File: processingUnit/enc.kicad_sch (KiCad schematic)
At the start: 14 parts, among them J305 Conn_01x04, SW201 ENC RST, U201 STM32F103Cx, Y201 8Mhz

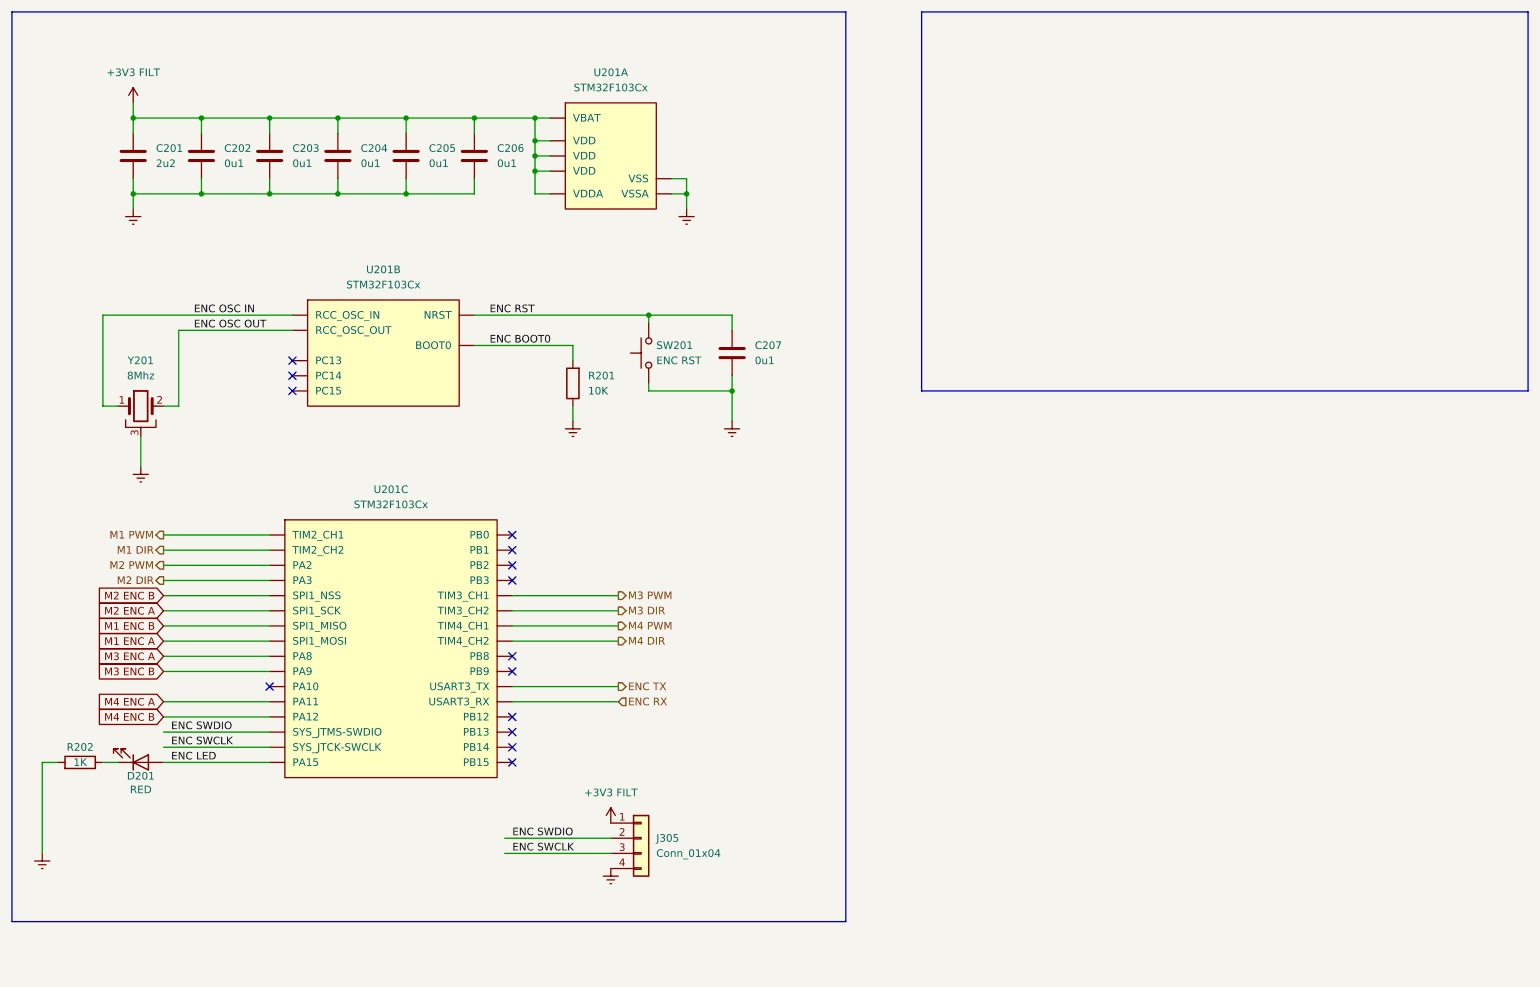
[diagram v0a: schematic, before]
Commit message: l3 might redo
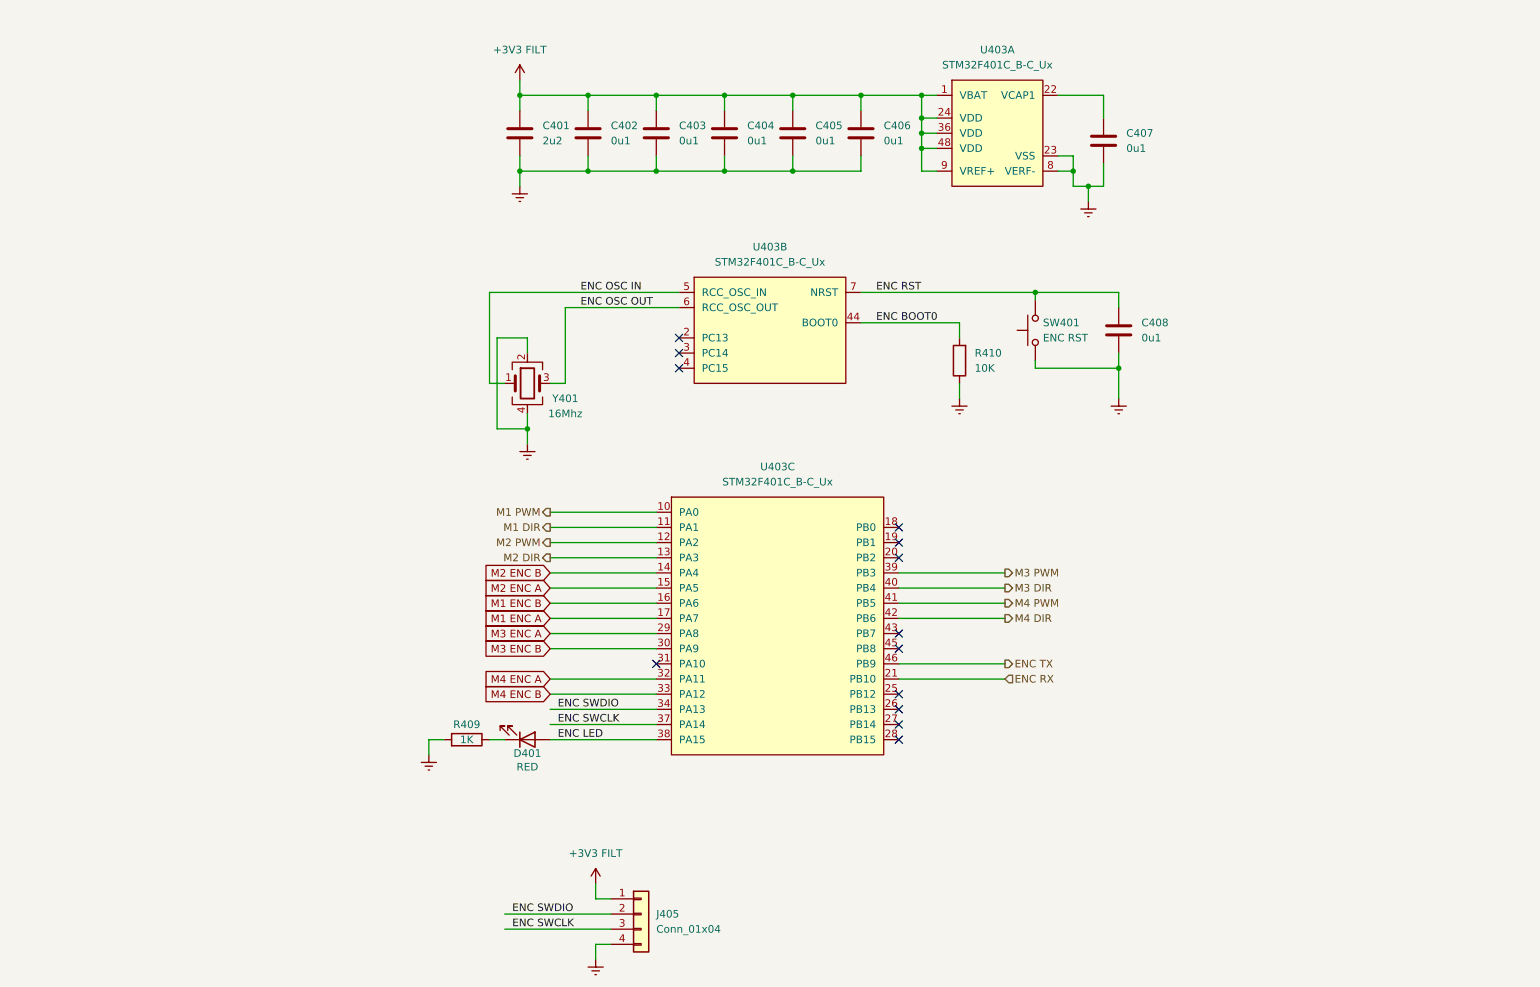
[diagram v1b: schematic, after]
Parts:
- removed U201: STM32F103Cx, Package_DFN_QFN:QFN-48-1EP_7x7mm_P0.5mm_EP5.6x5.6mm, symbol vincent:STM32F103Cx
- removed Y201: 8Mhz, Library:CSTCE8M00G52-R0, symbol Device:Crystal_GND3
- added C407: 0u1, Library:cap0603, symbol Device:C
- added U403: STM32F401C_B-C_Ux, Package_DFN_QFN:QFN-48-1EP_7x7mm_P0.5mm_EP5.6x5.6mm, symbol vincent:STM32F401C_B-C_Ux
- added Y401: 16Mhz, Library:CX3225SB16000D0FPLCC, symbol Device:Crystal_GND24
- renumbered C201 to C401, C202 to C402, C203 to C403, C204 to C404, C205 to C405, C206 to C406, C207 to C408, D201 to D401, J305 to J405, R202 to R409, R201 to R410, SW201 to SW401
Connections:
- net +3V3 FILT: now also U403.1 (VBAT), U403.24 (VDD), U403.36 (VDD), U403.48 (VDD), U403.9 (VREF+)
- net ENC BOOT0: now also U403.44 (BOOT0)
- net ENC LED: now also U403.38 (PA15)
- net ENC OSC IN: now also U403.5 (PH0), Y401.1
- net ENC OSC OUT: now also U403.6 (PH1), Y401.3
- net ENC RST: now also U403.7 (NRST)
- net ENC RX: now also U403.21 (PB10)
- net ENC SWCLK: now also U403.37 (PA14)
- net ENC SWDIO: now also U403.34 (PA13)
- net ENC TX: now also U403.46 (PB9)
- net GNDREF: now also C407.2, U403.23 (VSS), U403.35 (VSS), U403.47 (VSS), U403.49 (VSS), U403.8 (VERF-), Y401.2, Y401.4
- net M1 DIR: now also U403.11 (PA1)
- net M1 ENC A: now also U403.17 (PA7)
- net M1 ENC B: now also U403.16 (PA6)
- net M1 PWM: now also U403.10 (PA0)
- net M2 DIR: now also U403.13 (PA3)
- net M2 ENC A: now also U403.15 (PA5)
- net M2 ENC B: now also U403.14 (PA4)
- net M2 PWM: now also U403.12 (PA2)
- net M3 DIR: now also U403.40 (PB4)
- net M3 ENC A: now also U403.29 (PA8)
- net M3 ENC B: now also U403.30 (PA9)
- net M3 PWM: now also U403.39 (PB3)
- net M4 DIR: now also U403.42 (PB6)
- net M4 ENC A: now also U403.32 (PA11)
- net M4 ENC B: now also U403.33 (PA12)
- net M4 PWM: now also U403.41 (PB5)
- new net: C407.1, U403.22 (VCAP1)
- no-connect marks 14 -> 13
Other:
- moved on the sheet: C401, C402, C403, C404, C405, C406, C408, D401, J405, R409, R410, SW401
